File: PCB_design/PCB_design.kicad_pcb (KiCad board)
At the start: 2 copper layers, 59.7 x 59.7 mm, 48 parts, among them J10 Conn_01x01_Socket, J11 Conn_01x01_Socket, J2 Conn_01x04_Socket, J3 Conn_01x01_Socket, J4 Conn_01x02_Pin, J5 Conn_01x01_Socket, J6 Conn_01x01_Socket, J7 Conn_01x01_Socket, J8 Conn_01x01_Socket, J9 USB_C_Receptacle_PowerOnly_6P, Q1 FS8205A, U1 L298N, U2 L7805, U3 TP4056, U4 DW01A

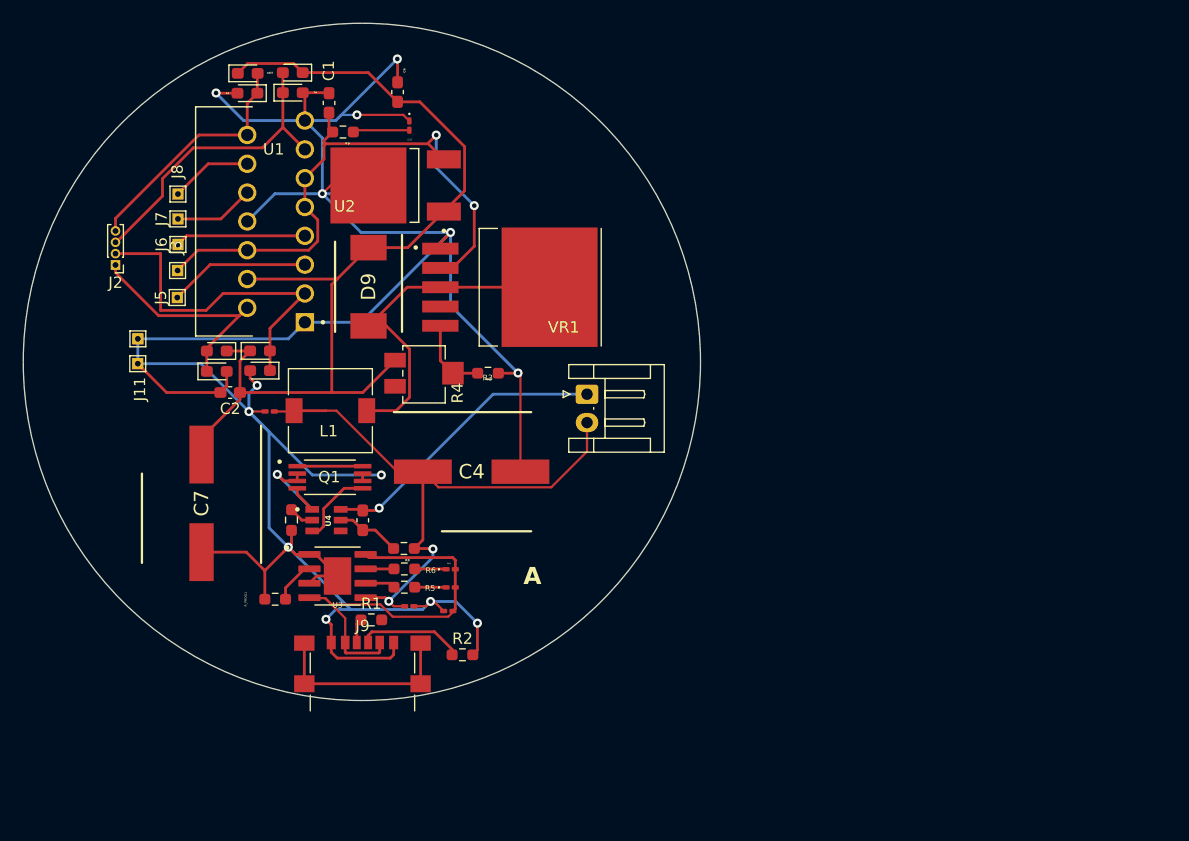
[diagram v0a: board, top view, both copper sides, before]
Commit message: Added PCB design pdf
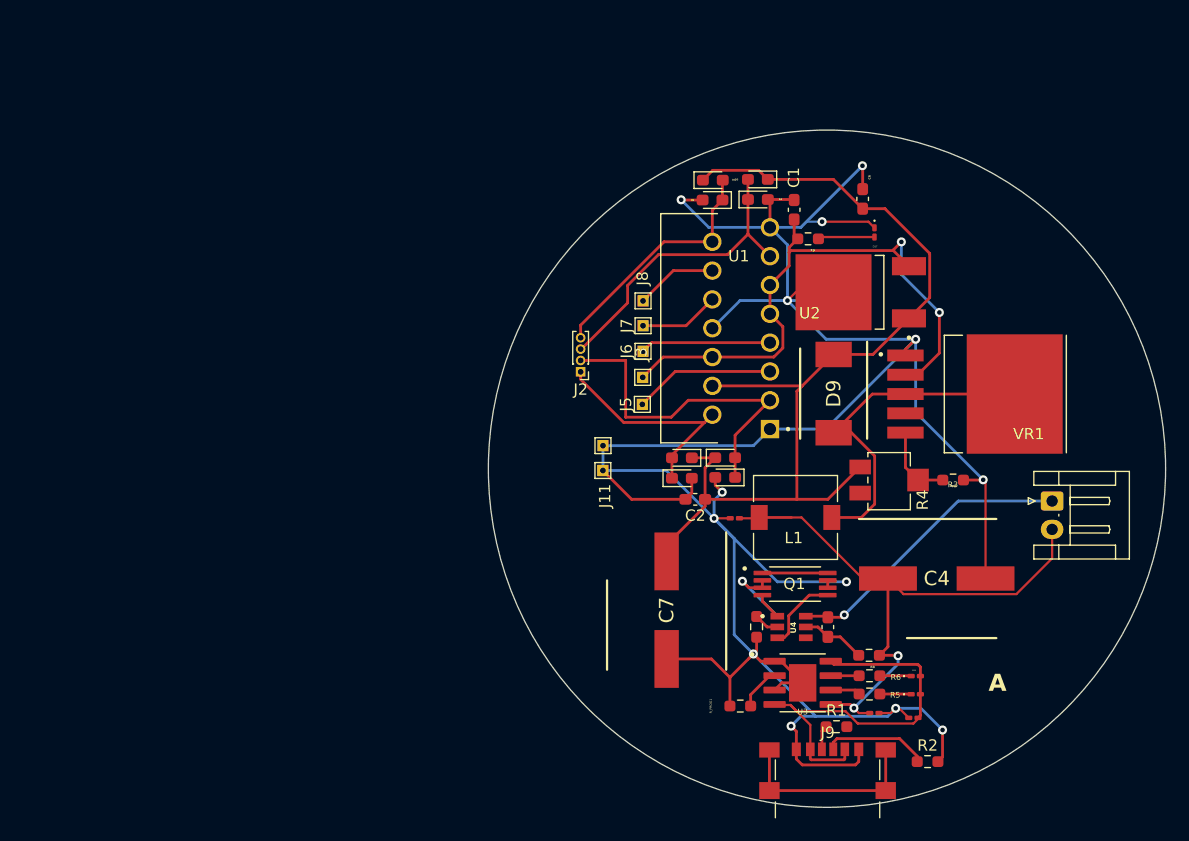
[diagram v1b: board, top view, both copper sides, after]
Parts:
- moved C1 42.1 mm to (99.2, 42.2)
- moved C10 42.1 mm to (102.1, 79.0)
- moved C4 42.1 mm to (111.7, 74.7)
- moved C5 42.1 mm to (93.9, 69.4)
- moved C6 42.1 mm to (105.2, 41.3)
- moved C9 42.1 mm to (106.2, 86.6)
- moved D1 42.1 mm to (92.0, 39.6)
- moved D10 42.1 mm to (109.9, 84.9)
- moved D11 42.1 mm to (109.9, 83.3)
- moved D17 42.1 mm to (106.2, 44.2)
- moved D3 42.1 mm to (96.0, 39.5)
- moved J11 42.1 mm to (82.3, 65.2)
- moved J4 42.1 mm to (121.9, 67.9)
- moved Q1 42.1 mm to (99.2, 75.2)
- moved R5 42.1 mm to (105.8, 84.9)
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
